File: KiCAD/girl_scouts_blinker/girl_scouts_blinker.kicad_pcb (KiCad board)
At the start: 2 copper layers, 71.1 x 43.2 mm, 18 parts, among them J1 AVR-ISP-6, SW1 SW_Push, SW2 SW_Push, SW3 SW_SPST, U1 ATtiny85-20P

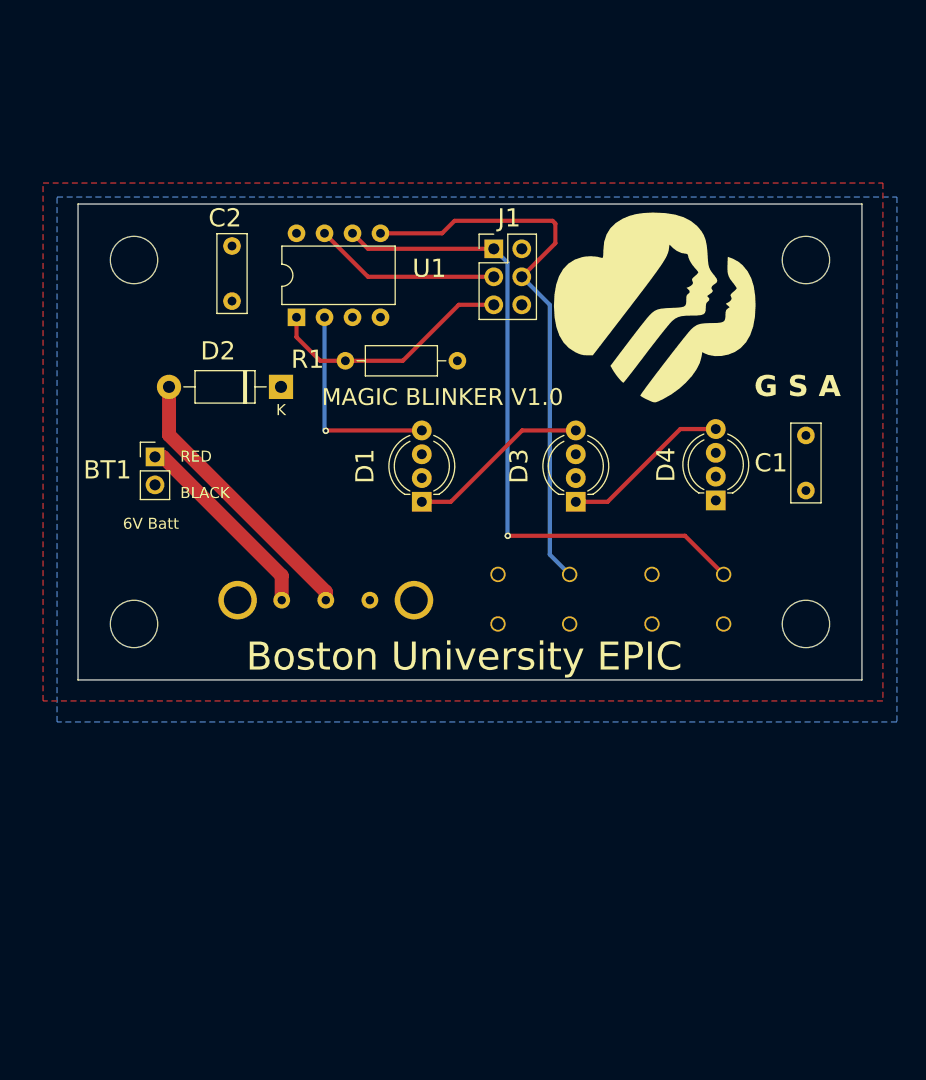
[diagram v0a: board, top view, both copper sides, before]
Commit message: layout v1.1 done?
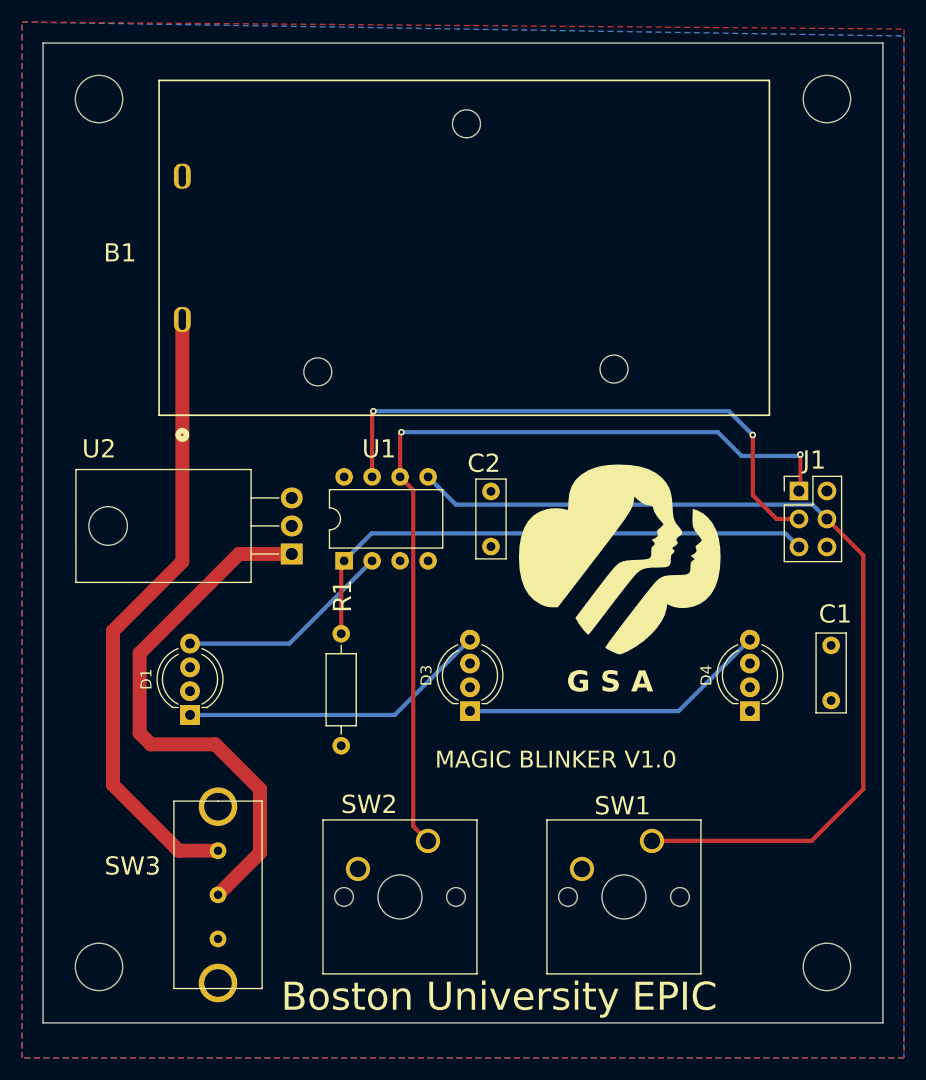
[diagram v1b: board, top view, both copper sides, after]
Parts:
- removed BT1: Battery, Connector_PinHeader_2.54mm:PinHeader_1x02_P2.54mm_Vertical
- removed D2: 1N4002, Diode_THT:D_DO-41_SOD81_P10.16mm_Horizontal
- added B1: BC9VPC, my_footprints:BC9VPC_MPD, F.Cu at (52.6, 53.7)
- added U2: LM7805_TO220, Package_TO_SOT_THT:TO-220-3_Horizontal_TabDown, F.Cu at (62.6, 74.9)
- D1, D3, D4: footprint LED_THT:LED_D5.0mm-4_RGB_Wide_Pins -> my_neopixel:LED_D5.0mm-4_RGB_Wide_Pins
- SW1, SW2: footprint push_sw:BTN-B3F-1000 -> my_cherry:SW_Cherry_MX_1.00u_PCB; moved to F.Cu
- SW3: moved to F.Cu
- moved H4 71.3 mm to (45.1, 112.4)
- moved H3 70.1 mm to (111.1, 112.4)
- moved R1 36.5 mm to (67.1, 92.3), turned to 90 degrees
- moved SW2 36.1 mm to (74.9, 101.0), turned to 0 degrees
- moved J1 35.3 mm to (108.6, 69.2)
- moved C2 32.4 mm to (80.6, 69.3)
- moved D1 28.6 mm to (53.3, 89.5)
- moved SW3 28.5 mm to (55.9, 105.9), turned to -90 degrees
- moved SW1 25.3 mm to (95.2, 101.0), turned to 0 degrees
- moved FID1 23.1 mm to (92.2, 75.3)
- moved U1 22.5 mm to (67.3, 75.6)
- moved D3 21.3 mm to (78.7, 89.2)
- moved D4 19.4 mm to (104.1, 89.2)
- moved C1 19.2 mm to (111.5, 83.2)
- moved H1 14.9 mm to (45.1, 33.7)
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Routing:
- net +6V: track 18.2 -> 56.8 mm
- net /SCK: track 17.0 -> 51.9 mm, vias 0 -> 2
- net /MOSI: track 51.3 -> 84.8 mm
- net /nRST: track 22.7 -> 49.5 mm
- net Net-(SW3-B): track 25.2 -> 49.0 mm
- net /MISO: track 61.0 -> 78.7 mm, vias 1 -> 2
- net Net-(D3-DOUT): track 15.4 -> 28.1 mm
- net Net-(D1-DOUT): track 16.7 -> 28.2 mm
- net Net-(D1-DIN): track 19.1 -> 19.6 mm, vias 1 -> 0
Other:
- board size 71.1 x 43.2 mm -> 76.2 x 88.9 mm
- board text removed: "6V Batt"
- board text removed: "BLACK"
- board text removed: "RED"
